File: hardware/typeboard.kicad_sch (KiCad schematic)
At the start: 0 parts

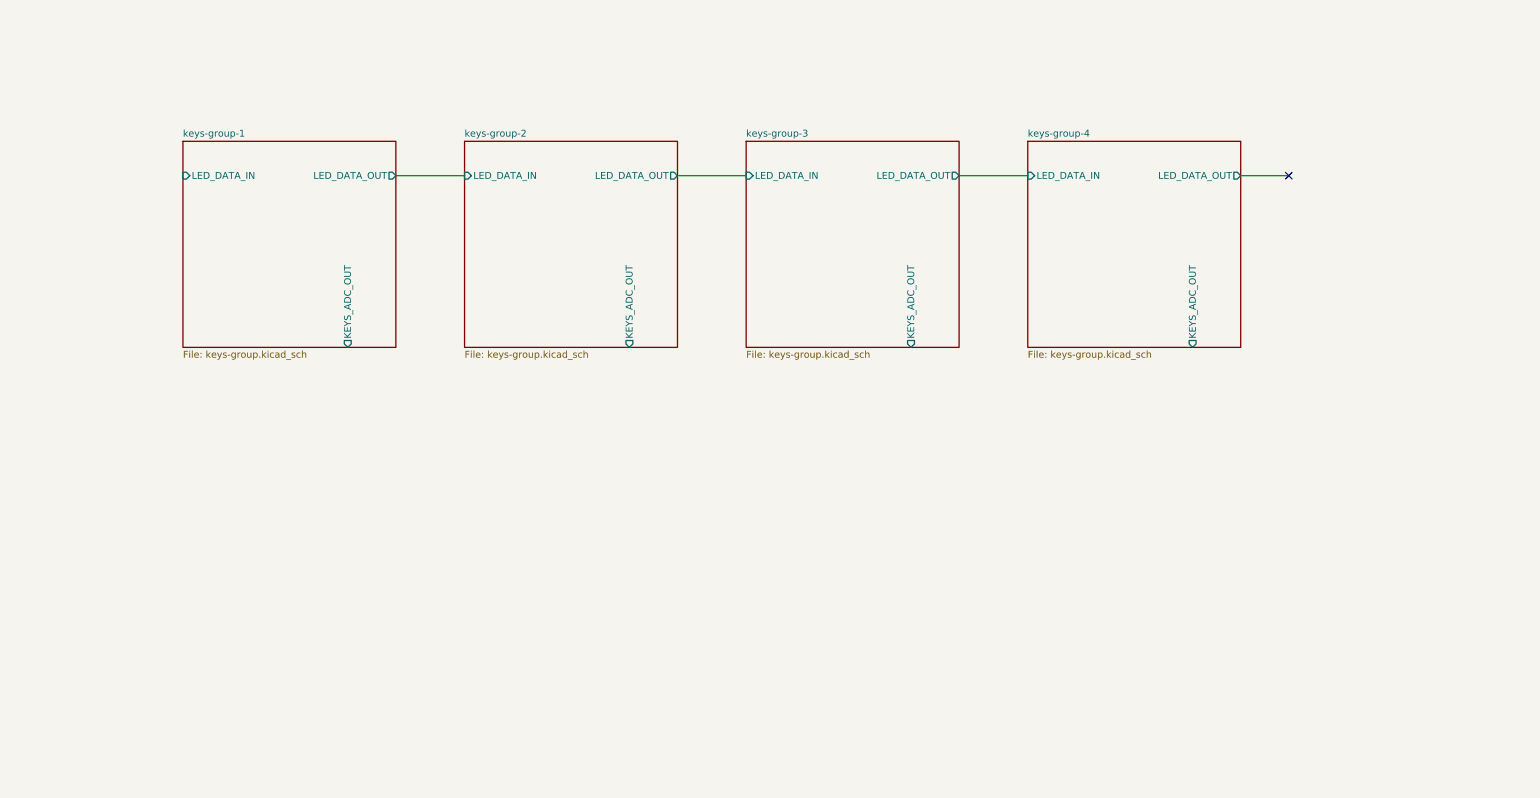
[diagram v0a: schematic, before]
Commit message: :construction: explode saki
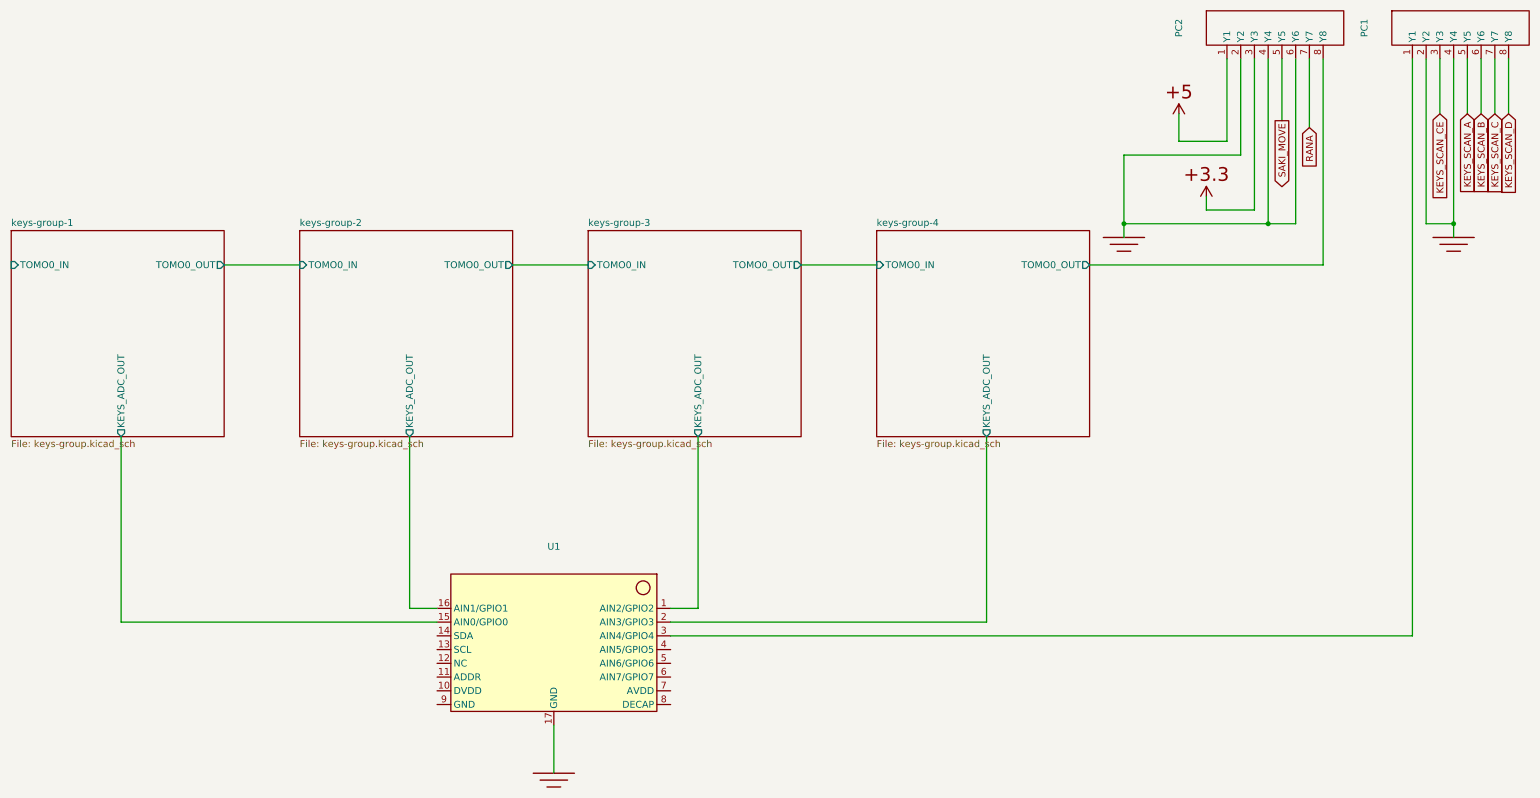
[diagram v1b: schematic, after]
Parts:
- added PC1, PC2: ~, KeysDock:POGOPIN-8P-HR, symbol components:POGOPIN-8P-HR
- added U1: ~, KeysDock:TLA2528, symbol components:TLA2528
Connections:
- net keys-group-1/KEYS_ADC_OUT: now also U1.15 (AIN0/GPIO0)
- net keys-group-2/KEYS_ADC_OUT: now also U1.16 (AIN1/GPIO1)
- net keys-group-3/KEYS_ADC_OUT: now also U1.1 (AIN2/GPIO2)
- net keys-group-4/KEYS_ADC_OUT: now also U1.2 (AIN3/GPIO3)
- new net: PC1.1 (Y1), U1.3 (AIN4/GPIO4)
- new net KEYS_SCAN_A: PC1.5 (Y5)
- new net KEYS_SCAN_B: PC1.6 (Y6)
- new net KEYS_SCAN_C: PC1.7 (Y7)
- new net KEYS_SCAN_CE: PC1.3 (Y3)
- new net KEYS_SCAN_D: PC1.8 (Y8)
- new net P,+3.3: PC2.3 (Y3)
- new net P,+5: PC2.1 (Y1)
- new net P,E: PC1.2 (Y2), PC1.4 (Y4), PC2.2 (Y2), PC2.4 (Y4), PC2.6 (Y6), U1.17 (GND)
- new net RANA: PC2.7 (Y7)
- new net SAKI_MOVE: PC2.5 (Y5)
- new net keys-group-4/TOMO0_OUT: PC2.8 (Y8)
- no-connect marks 1 -> 0
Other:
- sheet keys-group-1 ports: added TOMO0_IN, TOMO0_OUT; removed LED_DATA_IN, LED_DATA_OUT
- sheet keys-group-2 ports: added TOMO0_IN, TOMO0_OUT; removed LED_DATA_IN, LED_DATA_OUT
- sheet keys-group-3 ports: added TOMO0_IN, TOMO0_OUT; removed LED_DATA_IN, LED_DATA_OUT
- sheet keys-group-4 ports: added TOMO0_IN, TOMO0_OUT; removed LED_DATA_IN, LED_DATA_OUT
